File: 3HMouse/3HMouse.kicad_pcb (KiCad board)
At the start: 2 copper layers, 200 x 100 mm, 0 parts

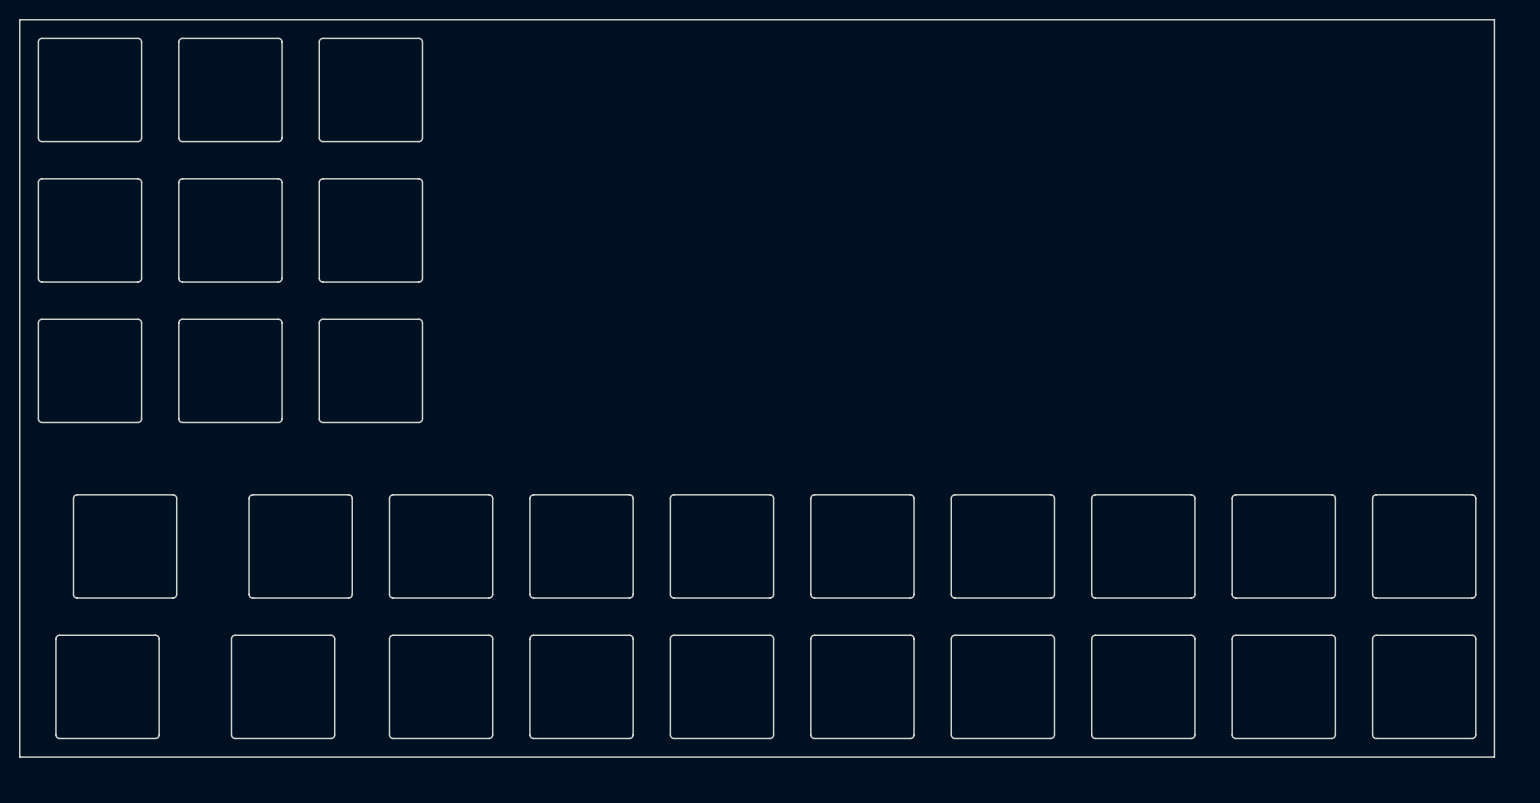
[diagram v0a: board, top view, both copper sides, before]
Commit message: v0.1.0
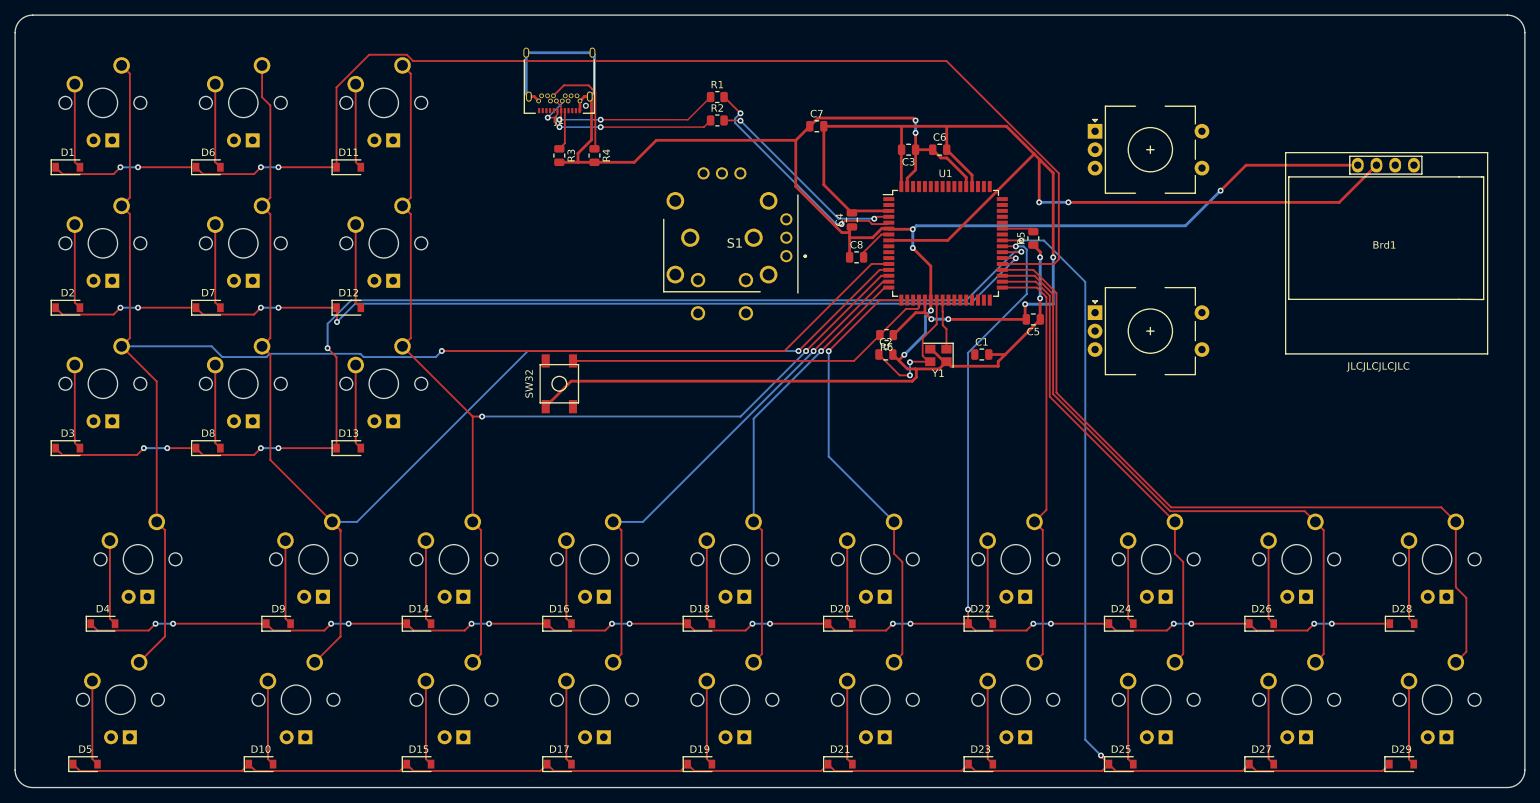
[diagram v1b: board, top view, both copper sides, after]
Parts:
- added Brd1: SSD1306, SSD1306:128x64OLED, F.Cu at (215.1, 60.3)
- added C1: 22pF, Capacitor_SMD:C_0805_2012Metric, F.Cu at (160.5, 75.4)
- added C2: 22pF, Capacitor_SMD:C_0805_2012Metric, F.Cu at (147.5, 75.4)
- added C3: 0.1uF, Capacitor_SMD:C_0805_2012Metric, F.Cu at (150.6, 47.6)
- added C4: 0.1uF, Capacitor_SMD:C_0805_2012Metric, F.Cu at (142.9, 57.1)
- added C5: 0.1uF, Capacitor_SMD:C_0805_2012Metric, F.Cu at (167.5, 70.6)
- added C6: 0.1uF, Capacitor_SMD:C_0805_2012Metric, F.Cu at (154.8, 47.6)
- added C7: 10uF, Capacitor_SMD:C_0805_2012Metric, F.Cu at (138.1, 44.5)
- added C8: 1uF, Capacitor_SMD:C_0805_2012Metric, F.Cu at (143.5, 62.2)
- added D1: D_Small, Diode_SMD:D_SOD-123, F.Cu at (36.5, 50.0)
- added D10: D_Small, Diode_SMD:D_SOD-123, F.Cu at (62.7, 131.0)
- added D11: D_Small, Diode_SMD:D_SOD-123, F.Cu at (74.6, 50.0)
- added D12: D_Small, Diode_SMD:D_SOD-123, F.Cu at (74.6, 69.1)
- added D13: D_Small, Diode_SMD:D_SOD-123, F.Cu at (74.6, 88.1)
- added D14: D_Small, Diode_SMD:D_SOD-123, F.Cu at (84.1, 111.9)
- added D15: D_Small, Diode_SMD:D_SOD-123, F.Cu at (84.1, 131.0)
- added D16: D_Small, Diode_SMD:D_SOD-123, F.Cu at (103.2, 111.9)
- added D17: D_Small, Diode_SMD:D_SOD-123, F.Cu at (103.2, 131.0)
- added D18: D_Small, Diode_SMD:D_SOD-123, F.Cu at (122.2, 111.9)
- added D19: D_Small, Diode_SMD:D_SOD-123, F.Cu at (122.2, 131.0)
- added D2: D_Small, Diode_SMD:D_SOD-123, F.Cu at (36.5, 69.1)
- added D20: D_Small, Diode_SMD:D_SOD-123, F.Cu at (141.3, 111.9)
- added D21: D_Small, Diode_SMD:D_SOD-123, F.Cu at (141.3, 131.0)
- added D22: D_Small, Diode_SMD:D_SOD-123, F.Cu at (160.3, 111.9)
- added D23: D_Small, Diode_SMD:D_SOD-123, F.Cu at (160.3, 131.0)
- added D24: D_Small, Diode_SMD:D_SOD-123, F.Cu at (179.4, 111.9)
- added D25: D_Small, Diode_SMD:D_SOD-123, F.Cu at (179.4, 131.0)
- added D26: D_Small, Diode_SMD:D_SOD-123, F.Cu at (198.4, 111.9)
- added D27: D_Small, Diode_SMD:D_SOD-123, F.Cu at (198.4, 131.0)
- added D28: D_Small, Diode_SMD:D_SOD-123, F.Cu at (217.5, 111.9)
- added D29: D_Small, Diode_SMD:D_SOD-123, F.Cu at (217.4, 131.0)
- added D3: D_Small, Diode_SMD:D_SOD-123, F.Cu at (36.5, 88.1)
- added D4: D_Small, Diode_SMD:D_SOD-123, F.Cu at (41.3, 111.9)
- added D5: D_Small, Diode_SMD:D_SOD-123, F.Cu at (38.9, 131.0)
- added D6: D_Small, Diode_SMD:D_SOD-123, F.Cu at (55.6, 50.0)
- added D7: D_Small, Diode_SMD:D_SOD-123, F.Cu at (55.6, 69.1)
- added D8: D_Small, Diode_SMD:D_SOD-123, F.Cu at (55.6, 88.1)
- added D9: D_Small, Diode_SMD:D_SOD-123, F.Cu at (65.1, 111.9)
- added J1: USB_C_Receptacle, Connector_USB:USB_C_Receptacle_Amphenol_12401548E4-2A, F.Cu at (103.2, 37.3)
- added R1: 22, Resistor_SMD:R_0805_2012Metric, F.Cu at (124.6, 40.5)
- added R2: 22, Resistor_SMD:R_0805_2012Metric, F.Cu at (124.6, 43.7)
- added R3: 5.1k, Resistor_SMD:R_0805_2012Metric, F.Cu at (103.2, 48.4)
- added R4: 5.1k, Resistor_SMD:R_0805_2012Metric, F.Cu at (108.0, 48.4)
- added R5: 10k, Resistor_SMD:R_0805_2012Metric, F.Cu at (167.5, 59.6)
- added R6: 10k, Resistor_SMD:R_0805_2012Metric, F.Cu at (147.6, 72.8)
- added S1: RKJXV122400R, SamacSys_Parts:RKJXV122400R, F.Cu at (134.0, 62.1)
- added SW1: CherryMX, MX_Only:MXOnly-1U, F.Cu at (41.3, 41.3)
- added SW10: CherryMX, MX_Only:MXOnly-1U, F.Cu at (67.5, 122.2)
- added SW11: CherryMX, MX_Only:MXOnly-1U, F.Cu at (79.4, 41.3)
- added SW12: CherryMX, MX_Only:MXOnly-1U, F.Cu at (79.4, 60.3)
- added SW13: CherryMX, MX_Only:MXOnly-1U, F.Cu at (79.4, 79.4)
- added SW14: CherryMX, MX_Only:MXOnly-1U, F.Cu at (88.9, 103.2)
- added SW15: CherryMX, MX_Only:MXOnly-1U, F.Cu at (88.9, 122.2)
- added SW16: CherryMX, MX_Only:MXOnly-1U, F.Cu at (108.0, 103.2)
- added SW17: CherryMX, MX_Only:MXOnly-1U, F.Cu at (108.0, 122.2)
- added SW18: CherryMX, MX_Only:MXOnly-1U, F.Cu at (127.0, 103.2)
- added SW19: CherryMX, MX_Only:MXOnly-1U, F.Cu at (127.0, 122.2)
- added SW2: CherryMX, MX_Only:MXOnly-1U, F.Cu at (41.3, 60.3)
- added SW20: CherryMX, MX_Only:MXOnly-1U, F.Cu at (146.1, 103.2)
- added SW21: CherryMX, MX_Only:MXOnly-1U, F.Cu at (146.1, 122.2)
- added SW22: CherryMX, MX_Only:MXOnly-1U, F.Cu at (165.1, 103.2)
- added SW23: CherryMX, MX_Only:MXOnly-1U, F.Cu at (165.1, 122.2)
- added SW24: CherryMX, MX_Only:MXOnly-1U, F.Cu at (184.2, 103.2)
- added SW25: CherryMX, MX_Only:MXOnly-1U, F.Cu at (184.2, 122.2)
- added SW26: CherryMX, MX_Only:MXOnly-1U, F.Cu at (203.2, 103.2)
- added SW27: CherryMX, MX_Only:MXOnly-1U, F.Cu at (203.2, 122.2)
- added SW28: CherryMX, MX_Only:MXOnly-1U, F.Cu at (222.2, 103.2)
- added SW29: CherryMX, MX_Only:MXOnly-1U, F.Cu at (222.2, 122.2)
- added SW3: CherryMX, MX_Only:MXOnly-1U, F.Cu at (41.3, 79.4)
- added SW30: RotaryEncoder, Keebio-Parts:RotaryEncoder_EC11, F.Cu at (183.4, 72.2)
- added SW31: RotaryEncoder, Keebio-Parts:RotaryEncoder_EC11, F.Cu at (183.4, 47.6)
- added SW32: SW_Push, random-keyboard-parts:SKQG-1155865, F.Cu at (103.2, 79.4)
- added SW4: CherryMX, MX_Only:MXOnly-1U, F.Cu at (46.0, 103.2)
- added SW5: CherryMX, MX_Only:MXOnly-1U, F.Cu at (43.7, 122.2)
- added SW6: CherryMX, MX_Only:MXOnly-1U, F.Cu at (60.3, 41.3)
- added SW7: CherryMX, MX_Only:MXOnly-1U, F.Cu at (60.3, 60.3)
- added SW8: CherryMX, MX_Only:MXOnly-1U, F.Cu at (60.3, 79.4)
- added SW9: CherryMX, MX_Only:MXOnly-1U, F.Cu at (69.8, 103.2)
- added U1: AT90USB1286-A, Package_QFP:TQFP-64_14x14mm_P0.8mm, F.Cu at (155.6, 60.3)
- added Y1: 16 MHz, Crystal:Crystal_SMD_3225-4Pin_3.2x2.5mm, F.Cu at (154.6, 75.5)
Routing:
- net GND: track 0.00 -> 313.1 mm, vias 0 -> 9
- net ROW4: track 0.00 -> 265.8 mm, vias 0 -> 2
- net ROW3: track 0.00 -> 240.7 mm, vias 0 -> 20
- net COL0: track 0.00 -> 197.0 mm, vias 0 -> 1
- net +5V: track 0.00 -> 193.3 mm, vias 0 -> 6
- net COL1: track 0.00 -> 178.4 mm, vias 0 -> 1
- net ROW0: track 0.00 -> 176.5 mm, vias 0 -> 4
- net ROW2: track 0.00 -> 157.8 mm, vias 0 -> 6
- net COL2: track 0.00 -> 152.0 mm, vias 0 -> 2
- net ROW1: track 0.00 -> 139.1 mm, vias 0 -> 6
- net COL9: track 0.00 -> 103.8 mm
- net COL8: track 0.00 -> 84.2 mm
- net COL3: track 0.00 -> 70.9 mm, vias 0 -> 1
- net COL7: track 0.00 -> 64.9 mm
- net COL4: track 0.00 -> 59.7 mm, vias 0 -> 1
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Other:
- board size 200 x 100 mm -> 204.8 x 104.8 mm
- board text added: "JLCJLCJLCJLC"
